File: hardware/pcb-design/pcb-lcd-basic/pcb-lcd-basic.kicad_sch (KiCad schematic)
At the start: 44 parts, among them J1 Conn_01x20_Pin, J2 Conn_01x20_Pin, J3 Conn_01x06_Pin, J4 Conn_01x06_Pin, U1 NE555D, U10 74HC86, U11 74HC86, U12 74HC86, U13 74HC86, U14 74HC86, U15 74HC86, U16 74HC86, U17 AMS1117-3.3, U2 74HC595, U3 74HC595, U4 74HC595, U5 74HC595, U6 74HC595, U7 74HC86, U8 74HC86, U9 74HC86

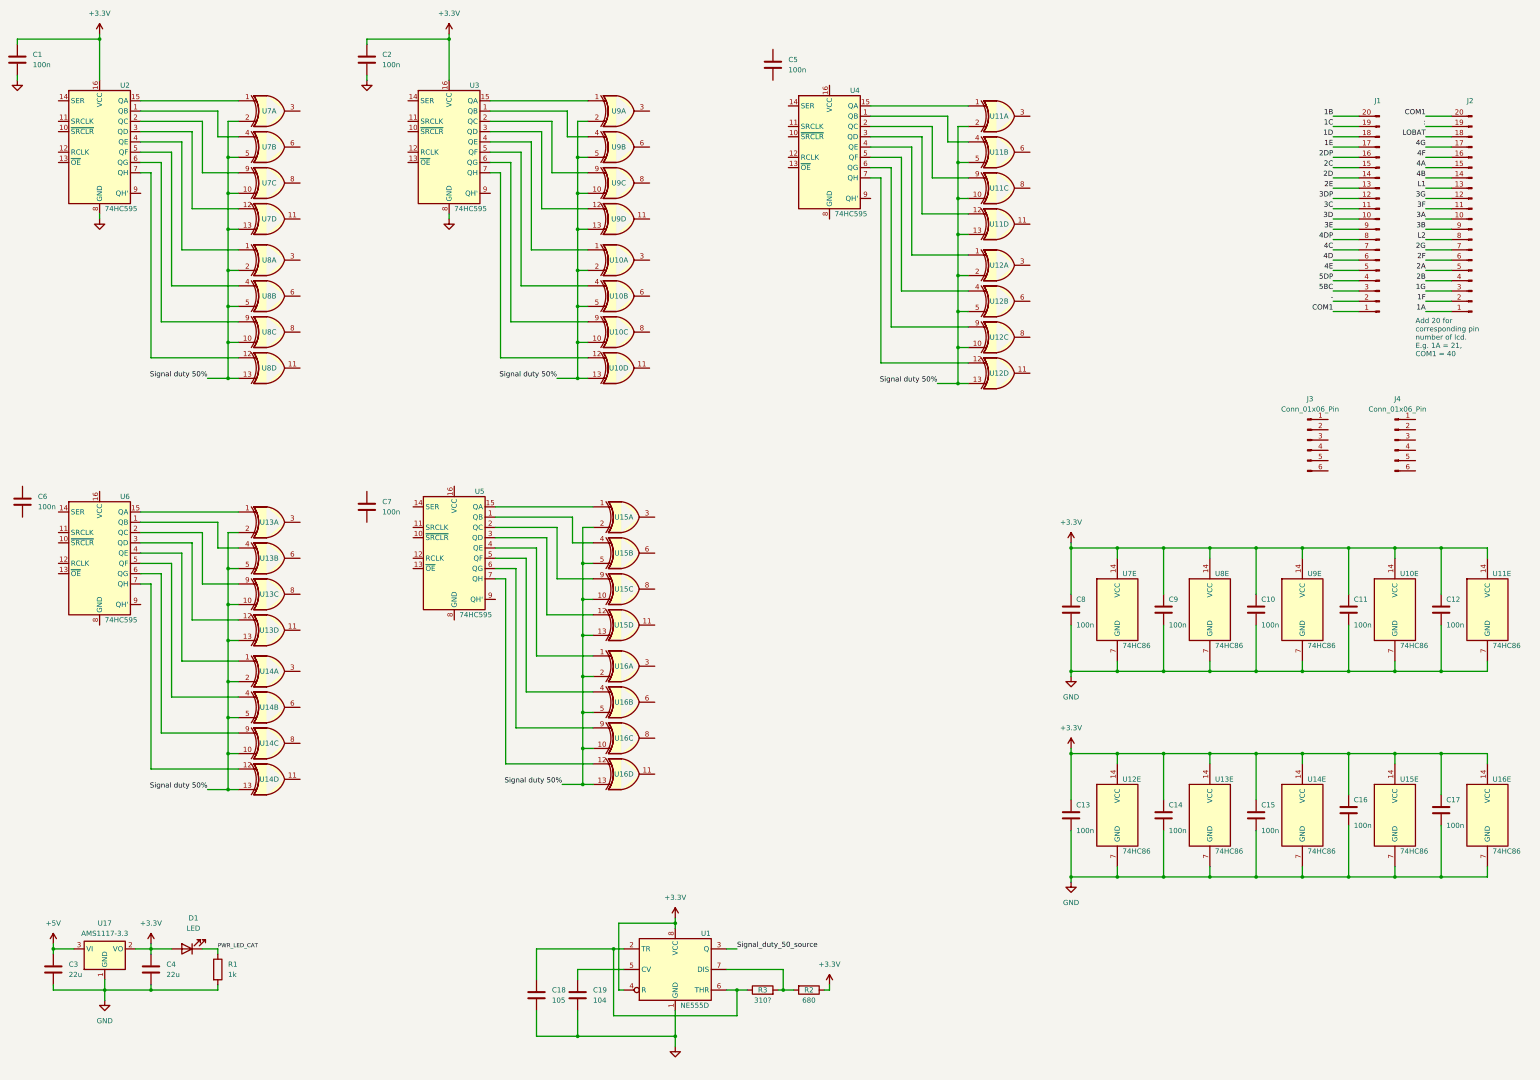
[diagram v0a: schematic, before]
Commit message: edit pcb schematic
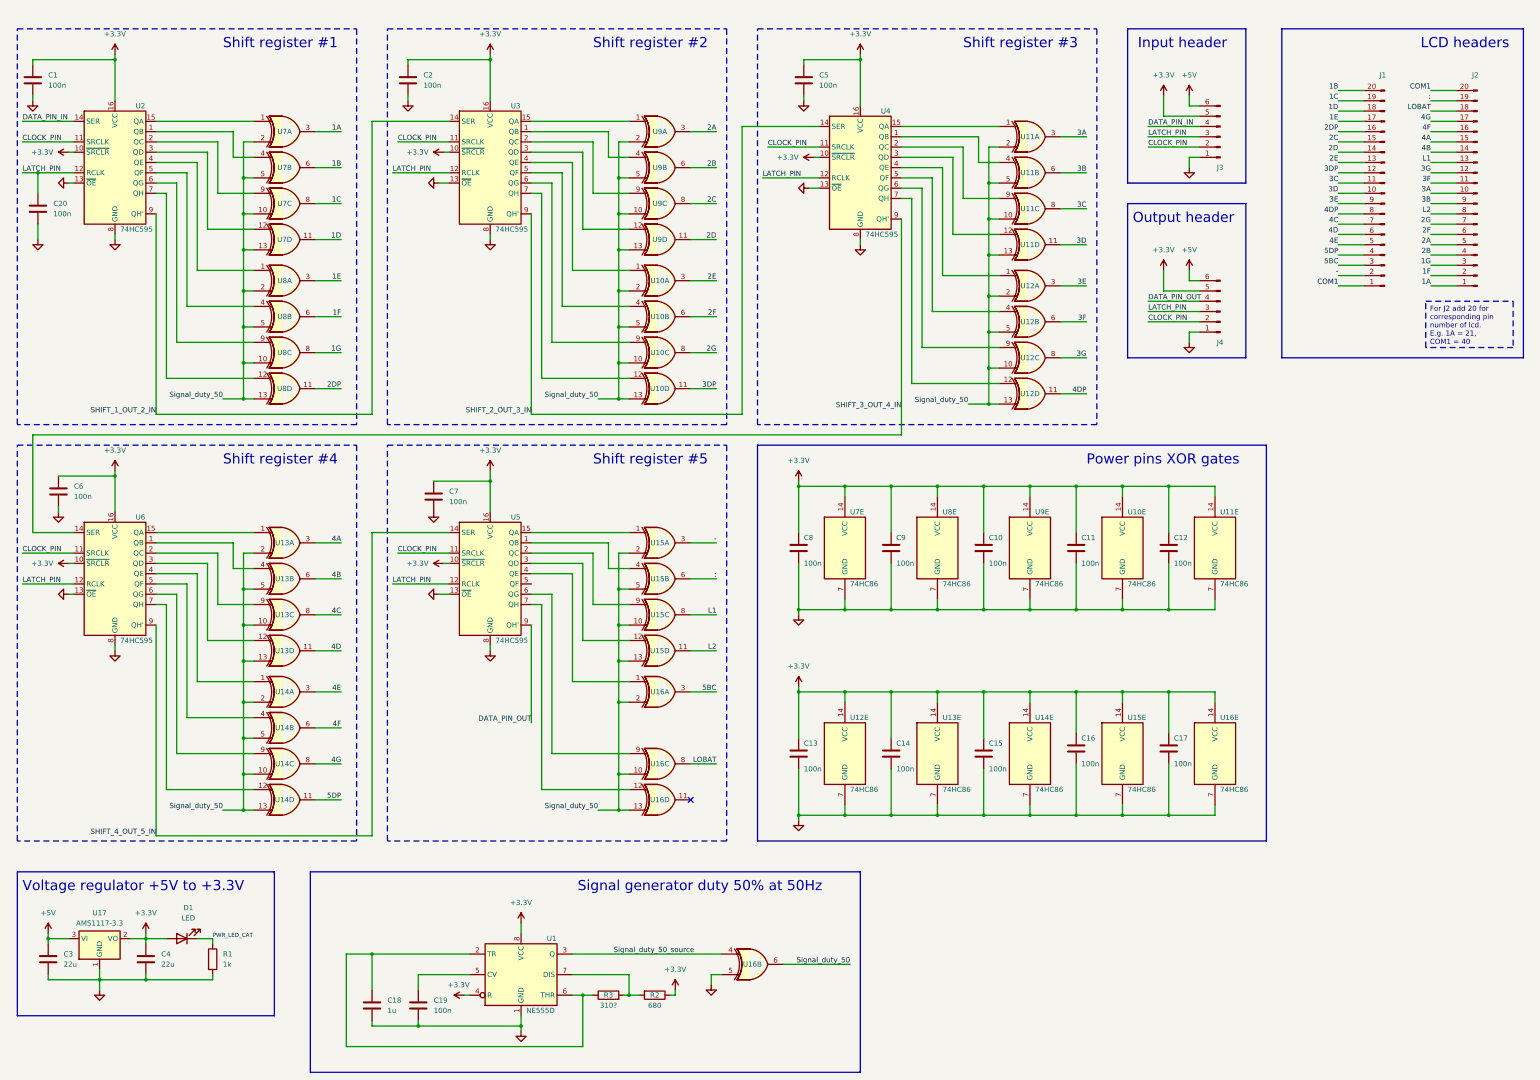
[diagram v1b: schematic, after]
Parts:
- added C20: 100n, symbol Device:C
- C18: value 105 -> 1u
- C19: value 104 -> 100n
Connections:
- net +3.3V: now also C5.1, C6.1, C7.1, J3.5 (Pin_5), J4.5 (Pin_5), U2.10 (~{SRCLR}), U3.10 (~{SRCLR}), U4.10 (~{SRCLR}), U4.16 (VCC), U5.10 (~{SRCLR}), U5.16 (VCC), U6.10 (~{SRCLR}), U6.16 (VCC)
- net +5V: now also J3.6 (Pin_6), J4.6 (Pin_6)
- net -: now also U15.3
- net 1A: now also U7.3
- net 1B: now also U7.6
- net 1C: now also U7.8
- net 1D: now also U7.11
- net 1E: now also U8.3
- net 1F: now also U8.6
- net 1G: now also U8.8
- net 2A: now also U9.3
- net 2B: now also U9.6
- net 2C: now also U9.8
- net 2D: now also U9.11
- net 2DP: now also U8.11
- net 2E: now also U10.3
- net 2F: now also U10.6
- net 2G: now also U10.8
- net 3A: now also U11.3
- net 3B: now also U11.6
- net 3C: now also U11.8
- net 3D: now also U11.11
- net 3DP: now also U10.11
- net 3E: now also U12.3
- net 3F: now also U12.6
- net 3G: now also U12.8
- net 4A: now also U13.3
- net 4B: now also U13.6
- net 4C: now also U13.8
- net 4D: now also U13.11
- net 4DP: now also U12.11
- net 4E: now also U14.3
- net 4F: now also U14.6
- net 4G: now also U14.8
- net 5BC: now also U16.3
- net 5DP: now also U14.11
- net :: now also U15.6
- net GND: now also C5.2, C6.2, C7.2, J3.1 (Pin_1), J4.1 (Pin_1), U16.5, U2.13 (~{OE}), U3.13 (~{OE}), U4.13 (~{OE}), U4.8 (GND), U5.13 (~{OE}), U5.8 (GND), U6.13 (~{OE}), U6.8 (GND), C20.2
- net L1: now also U15.8
- net L2: now also U15.11
- net LOBAT: now also U16.8
- net Signal_duty_50_source: now also U16.4
- net CLOCK_PIN: now reaches U4.11 (SRCLK)
- net CLOCK_PIN: now also J3.2 (Pin_2), J4.2 (Pin_2), U2.11 (SRCLK), U3.11 (SRCLK), U5.11 (SRCLK), U6.11 (SRCLK)
- net LATCH_PIN: now reaches U4.12 (RCLK)
- net LATCH_PIN: now also J3.3 (Pin_3), J4.3 (Pin_3), U2.12 (RCLK), U3.12 (RCLK), U5.12 (RCLK), U6.12 (RCLK), C20.1
- net SHIFT_2_OUT_3_IN: now reaches U4.14 (SER)
- net SHIFT_2_OUT_3_IN: now also U3.9 (QH')
- net SHIFT_3_OUT_4_IN: now reaches U4.9 (QH')
- net SHIFT_3_OUT_4_IN: now also U6.14 (SER)
- net SHIFT_1_OUT_2_IN: now reaches U3.14 (SER)
- net SHIFT_1_OUT_2_IN: now also U2.9 (QH')
- net SHIFT_4_OUT_5_IN: now reaches U6.9 (QH')
- net SHIFT_4_OUT_5_IN: now also U5.14 (SER)
- net DATA_PIN_IN: now reaches J3.4 (Pin_4)
- net DATA_PIN_IN: now also U2.14 (SER)
- net at U5.5 (QF): no longer U16.4
- net DATA_PIN_OUT: now reaches U5.9 (QH')
- net DATA_PIN_OUT: now also J4.4 (Pin_4)
- net Signal_duty_50: now reaches U16.6
- net Signal_duty_50: now also U10.10, U10.13, U10.2, U10.5, U11.10, U11.13, U11.2, U11.5, U12.10, U12.13, U12.2, U12.5, U13.10, U13.13, U13.2, U13.5, U14.10, U14.13, U14.2, U14.5, U15.10, U15.13, U15.2, U15.5, U16.10, U16.13, U16.2, U7.10, U7.13, U7.2, U7.5, U8.10, U8.13, U8.2, U8.5, U9.10, U9.13, U9.2, U9.5
- removed net Signal duty 50%: U10.10, U10.13, U10.2, U10.5, U11.10, U11.13, U11.2, U11.5, U12.10, U12.13, U12.2, U12.5, U13.10, U13.13, U13.2, U13.5, U14.10, U14.13, U14.2, U14.5, U15.10, U15.13, U15.2, U15.5, U16.10, U16.13, U16.2, U16.5, U7.10, U7.13, U7.2, U7.5, U8.10, U8.13, U8.2, U8.5, U9.10, U9.13, U9.2, U9.5
- no-connect marks 0 -> 1
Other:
- note added: "Input header"
- note added: "LCD headers"
- note added: "Output header"
- note added: "Power pins XOR gates"
- note added: "Shift register #1"
- note added: "Shift register #2"
- note added: "Shift register #3"
- note added: "Shift register #4"
- note added: "Shift register #5"
- note added: "Signal generator duty 50% at 50Hz"
- note added: "Voltage regulator +5V to +3.3V"
- note removed: "Add 20 for corresponding pin number of lcd. E.g. 1A = 21, COM1 = 40"
- moved on the sheet: C1, C10, C11, C12, C13, C14, C15, C16, C17, C18, C19, C2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
